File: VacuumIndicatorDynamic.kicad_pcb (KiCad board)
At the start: 2 copper layers, 151.2 x 100.4 mm, 105 parts, among them J1 Conn_01x02_Male, J2 Conn_01x03_Male, J3 Conn_01x03_Male, J4 Conn_01x03_Male, SW1 SW_DIP_x01, SW2 SW_DIP_x01, SW3 SW_DIP_x01, SW4 SW_DIP_x01, U1 AP1117-25, U2 YAAJ_BluePill

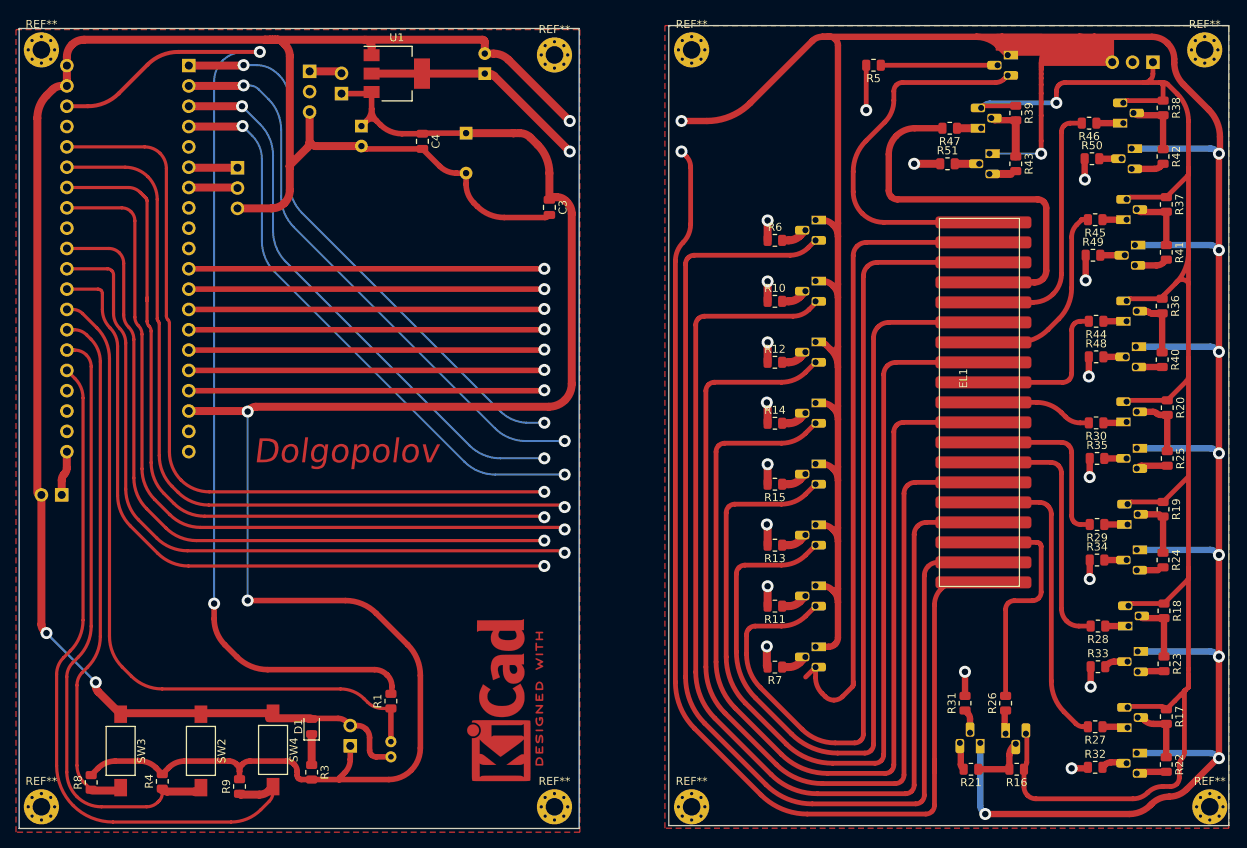
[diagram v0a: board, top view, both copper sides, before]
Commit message: major pcb update
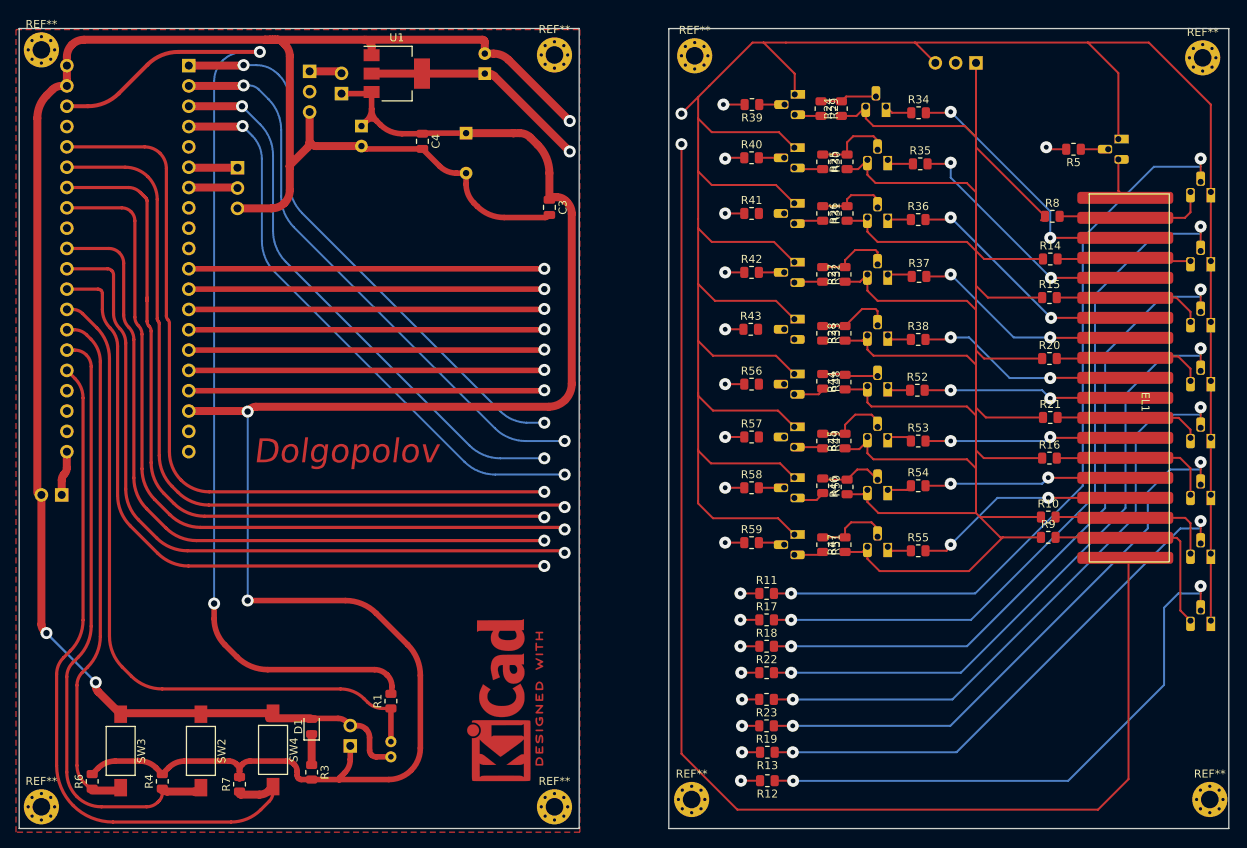
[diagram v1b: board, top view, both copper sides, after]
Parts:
- added R52: 510, Resistor_SMD:R_0805_2012Metric, F.Cu at (138.1, 68.6)
- added R53: 510, Resistor_SMD:R_0805_2012Metric, F.Cu at (138.2, 74.9)
- added R54: 510, Resistor_SMD:R_0805_2012Metric, F.Cu at (138.2, 80.5)
- added R55: 510, Resistor_SMD:R_0805_2012Metric, F.Cu at (138.2, 88.6)
- added R56: 4.7k, Resistor_SMD:R_0805_2012Metric, F.Cu at (117.3, 67.8)
- added R57: 4.7k, Resistor_SMD:R_0805_2012Metric, F.Cu at (117.3, 74.4)
- added R58: 4.7k, Resistor_SMD:R_0805_2012Metric, F.Cu at (117.3, 80.8)
- added R59: 4.7k, Resistor_SMD:R_0805_2012Metric, F.Cu at (117.3, 87.6)
- R10, R14, R15, R16, R20, R31, R32, R33, R48, R49, R50, R51: value 4.7k -> 47k
- R22, R23, R24, R25, R40, R41, R42, R43: value 47k -> 4.7k
- R26, R27, R28, R44, R45, R46, R47: value 510 -> 4.7k
- R29, R30: value 510 -> 47k
- R34, R35, R36, R37, R38: value 4.7k -> 510
- R6, R7: value 4.7k -> 10k
- R8, R9: value 10k -> 47k
- moved R8 139.4 mm to (154.9, 46.8), turned to 0 degrees
- moved R6 108.9 mm to (34.9, 117.5), turned to 90 degrees
- moved R9 105.8 mm to (154.4, 87.0), turned to 0 degrees
- moved VT16 86.9 mm to (122.7, 38.3)
- moved VT15 84.3 mm to (122.7, 31.6), turned to -90 degrees
- moved VT10 79.8 mm to (134.2, 33.1), turned to 180 degrees
- moved VT11 77.0 mm to (134.4, 39.8), turned to 180 degrees
- moved VT17 70.6 mm to (122.7, 45.2)
- moved R32 70.4 mm to (126.2, 54.1), turned to -90 degrees
- moved R24 69.3 mm to (128.6, 33.4), turned to 90 degrees
- moved R7 68.5 mm to (53.3, 117.8), turned to 90 degrees
- moved R27 64.6 mm to (129.0, 54.1), turned to 90 degrees
- moved R26 64.3 mm to (129.3, 46.5)
- moved VT5 63.9 mm to (174.8, 52.4), turned to 180 degrees
- moved R31 63.8 mm to (126.2, 46.5), turned to -90 degrees
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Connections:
- EL1 pad 1: +2V5 -> Net-(EL1-Pad1)
- EL1 pad 12: Net-(EL1-Pad12) -> /S_OUT_1
- EL1 pad 13: Net-(EL1-Pad13) -> /S_OUT_2
- EL1 pad 14: Net-(EL1-Pad14) -> /S_OUT_3
- EL1 pad 15: Net-(EL1-Pad15) -> /S_OUT_4
- EL1 pad 16: Net-(EL1-Pad16) -> /S_OUT_5
- EL1 pad 17: Net-(EL1-Pad17) -> /S_OUT_6
- EL1 pad 18: Net-(EL1-Pad18) -> /S_OUT_7
- EL1 pad 19: Net-(EL1-Pad19) -> /S_OUT_8
- EL1 pad 2: Net-(EL1-Pad2) -> +2V5
- R10 pad 1: /K2 -> +24V
- R10 pad 2: Net-(R10-Pad2) -> /S_OUT_7
- R11 pad 1: Net-(R11-Pad1) -> /S1
- R11 pad 2: /K7 -> Net-(R11-Pad2)
- R12 pad 1: /K3 -> Net-(R12-Pad1)
- R12 pad 2: Net-(R12-Pad2) -> /S8
- R13 pad 2: /K6 -> /S7
- R14 pad 1: /K4 -> +24V
- R14 pad 2: Net-(R14-Pad2) -> /S_OUT_2
- R15 pad 1: Net-(R15-Pad1) -> +24V
- R15 pad 2: /K5 -> /S_OUT_3
- R16 pad 2: Net-(R16-Pad2) -> /S_OUT_6
- R17 pad 1: +24V -> /S2
- R18 pad 1: +24V -> /S3
- R19 pad 1: +24V -> Net-(R19-Pad1)
- R19 pad 2: Net-(R19-Pad2) -> /S6
- R20 pad 2: Net-(R20-Pad2) -> /S_OUT_4
- R21 pad 1: Net-(R16-Pad2) -> +24V
- R21 pad 2: Net-(R21-Pad2) -> /S_OUT_5
- R22 pad 1: Net-(R17-Pad2) -> /S4
- R23 pad 1: Net-(R18-Pad2) -> Net-(R23-Pad1)
- R23 pad 2: Net-(R23-Pad2) -> /S5
- R24 pad 1: Net-(R19-Pad2) -> +24V
- R25 pad 1: Net-(R20-Pad2) -> +24V
- R26 pad 1: Net-(R26-Pad1) -> +24V
- R26 pad 2: /A1 -> Net-(R26-Pad2)
- R27 pad 1: Net-(R27-Pad1) -> +24V
- R27 pad 2: /A2 -> Net-(R27-Pad2)
- R28 pad 1: Net-(R28-Pad1) -> +24V
- R28 pad 2: /A3 -> Net-(R28-Pad2)
- R29 pad 1: Net-(R29-Pad1) -> Net-(R24-Pad2)
- R29 pad 2: /A4 -> Net-(R29-Pad2)
- R30 pad 1: Net-(R30-Pad1) -> Net-(R25-Pad2)
- R30 pad 2: /A5 -> Net-(R30-Pad2)
- R31 pad 1: Net-(R31-Pad1) -> Net-(R26-Pad2)
- R31 pad 2: /AU1 -> Net-(R31-Pad2)
- R32 pad 1: /AU2 -> Net-(R27-Pad2)
- R33 pad 1: /AU3 -> Net-(R28-Pad2)
- R34 pad 1: /AU4 -> Net-(R34-Pad1)
- R34 pad 2: Net-(R34-Pad2) -> /A1
- R35 pad 1: /AU5 -> Net-(R35-Pad1)
- R35 pad 2: Net-(R35-Pad2) -> /A2
- R36 pad 1: +24V -> Net-(R36-Pad1)
- R36 pad 2: Net-(R36-Pad2) -> /A3
- R37 pad 1: +24V -> Net-(R37-Pad1)
- R37 pad 2: Net-(R37-Pad2) -> /A4
- R38 pad 1: +24V -> Net-(R38-Pad1)
- R38 pad 2: Net-(R38-Pad2) -> /A5
- R39 pad 1: +24V -> Net-(R39-Pad1)
- R39 pad 2: Net-(R39-Pad2) -> /AU1
- R40 pad 1: Net-(R36-Pad2) -> /AU2
- R41 pad 1: Net-(R37-Pad2) -> /AU3
- R42 pad 1: Net-(R38-Pad2) -> /AU4
- R43 pad 1: Net-(R39-Pad2) -> /AU5
- R44 pad 1: Net-(R44-Pad1) -> +24V
- R44 pad 2: /A6 -> Net-(R44-Pad2)
- R45 pad 1: Net-(R45-Pad1) -> +24V
- R45 pad 2: /A7 -> Net-(R45-Pad2)
- R46 pad 1: Net-(R46-Pad1) -> +24V
- R46 pad 2: /A8 -> Net-(R46-Pad2)
- R47 pad 1: Net-(R47-Pad1) -> +24V
- R47 pad 2: /A9 -> Net-(R47-Pad2)
- R48 pad 1: /AU6 -> Net-(R44-Pad2)
- R49 pad 1: /AU7 -> Net-(R45-Pad2)
- R50 pad 1: /AU8 -> Net-(R46-Pad2)
- R51 pad 1: /AU9 -> Net-(R47-Pad2)
- R6 pad 1: /K1 -> /BTN3
- R6 pad 2: Net-(R6-Pad2) -> +5V
- R7 pad 1: Net-(R7-Pad1) -> /BTN1
- R7 pad 2: /K8 -> +5V
- R8 pad 1: /BTN3 -> +24V
- R8 pad 2: +5V -> /S_OUT_1
- R9 pad 1: /BTN1 -> +24V
- R9 pad 2: +5V -> /S_OUT_8
- U2 pad 1: /K3 -> /S3
- U2 pad 11: /AU9 -> /AU1
- U2 pad 12: /AU8 -> /AU2
- U2 pad 13: /AU7 -> /AU3
- U2 pad 14: /AU6 -> /AU4
- U2 pad 16: /AU4 -> /AU6
- U2 pad 17: /AU3 -> /AU7
- U2 pad 2: /K4 -> /S4
- U2 pad 29: /K8 -> /S8
- U2 pad 3: /K5 -> /S5
- U2 pad 30: /K7 -> /S7
- U2 pad 33: /AU1 -> /AU9
- U2 pad 34: /AU2 -> /AU8
- U2 pad 35: /K1 -> /S1
- U2 pad 36: /K2 -> /S2
- U2 pad 4: /K6 -> /S6
- VT1 pad 3: Net-(EL1-Pad2) -> Net-(EL1-Pad1)
- VT10 pad 1: Net-(R26-Pad1) -> Net-(R34-Pad1)
- VT10 pad 2: Net-(R16-Pad2) -> Net-(R24-Pad2)
- VT11 pad 1: Net-(R27-Pad1) -> Net-(R35-Pad1)
- VT11 pad 2: Net-(R17-Pad2) -> Net-(R25-Pad2)
- VT12 pad 1: Net-(R28-Pad1) -> Net-(R36-Pad1)
- VT12 pad 2: Net-(R18-Pad2) -> Net-(R26-Pad2)
- VT13 pad 1: Net-(R29-Pad1) -> Net-(R37-Pad1)
- VT13 pad 2: Net-(R19-Pad2) -> Net-(R27-Pad2)
- VT14 pad 1: Net-(R30-Pad1) -> Net-(R38-Pad1)
- VT14 pad 2: Net-(R20-Pad2) -> Net-(R28-Pad2)
- VT15 pad 2: Net-(R31-Pad1) -> Net-(R39-Pad1)
- VT15 pad 3: Net-(R21-Pad2) -> Net-(R29-Pad2)
- VT16 pad 2: Net-(R32-Pad2) -> Net-(R40-Pad2)
- VT16 pad 3: Net-(R22-Pad2) -> Net-(R30-Pad2)
- VT17 pad 2: Net-(R33-Pad2) -> Net-(R41-Pad2)
- VT17 pad 3: Net-(R23-Pad2) -> Net-(R31-Pad2)
- VT18 pad 2: Net-(R34-Pad2) -> Net-(R42-Pad2)
- VT18 pad 3: Net-(R24-Pad2) -> Net-(R32-Pad2)
- VT19 pad 2: Net-(R35-Pad2) -> Net-(R43-Pad2)
- VT19 pad 3: Net-(R25-Pad2) -> Net-(R33-Pad2)
- VT2 pad 2: Net-(R6-Pad2) -> Net-(R11-Pad2)
- VT2 pad 3: Net-(EL1-Pad12) -> /S_OUT_1
- VT20 pad 1: Net-(R44-Pad1) -> Net-(R52-Pad1)
- VT20 pad 2: Net-(R36-Pad2) -> Net-(R44-Pad2)
- VT21 pad 1: Net-(R45-Pad1) -> Net-(R53-Pad1)
- VT21 pad 2: Net-(R37-Pad2) -> Net-(R45-Pad2)
- VT22 pad 1: Net-(R46-Pad1) -> Net-(R54-Pad1)
- VT22 pad 2: Net-(R38-Pad2) -> Net-(R46-Pad2)
- VT23 pad 1: Net-(R47-Pad1) -> Net-(R55-Pad1)
- VT23 pad 2: Net-(R39-Pad2) -> Net-(R47-Pad2)
- VT24 pad 2: Net-(R48-Pad2) -> Net-(R56-Pad2)
- VT24 pad 3: Net-(R40-Pad2) -> Net-(R48-Pad2)
- VT25 pad 2: Net-(R49-Pad2) -> Net-(R57-Pad2)
- VT25 pad 3: Net-(R41-Pad2) -> Net-(R49-Pad2)
- VT26 pad 2: Net-(R50-Pad2) -> Net-(R58-Pad2)
- VT26 pad 3: Net-(R42-Pad2) -> Net-(R50-Pad2)
- VT27 pad 2: Net-(R51-Pad2) -> Net-(R59-Pad2)
- VT27 pad 3: Net-(R43-Pad2) -> Net-(R51-Pad2)
- VT3 pad 2: Net-(R7-Pad1) -> Net-(R12-Pad1)
- VT3 pad 3: Net-(EL1-Pad19) -> /S_OUT_8
- VT4 pad 2: Net-(R10-Pad2) -> Net-(R13-Pad1)
- VT4 pad 3: Net-(EL1-Pad13) -> /S_OUT_7
- VT5 pad 2: Net-(R11-Pad1) -> Net-(R17-Pad2)
- VT5 pad 3: Net-(EL1-Pad18) -> /S_OUT_2
- VT6 pad 2: Net-(R12-Pad2) -> Net-(R18-Pad2)
- VT6 pad 3: Net-(EL1-Pad14) -> /S_OUT_3
- VT7 pad 2: Net-(R13-Pad1) -> Net-(R19-Pad1)
- VT7 pad 3: Net-(EL1-Pad17) -> /S_OUT_6
- VT8 pad 2: Net-(R14-Pad2) -> Net-(R22-Pad2)
- VT8 pad 3: Net-(EL1-Pad15) -> /S_OUT_4
- VT9 pad 2: Net-(R15-Pad1) -> Net-(R23-Pad1)
- VT9 pad 3: Net-(EL1-Pad16) -> /S_OUT_5
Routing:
- net Net-(EL1-Pad12): track 138.9 -> 0.00 mm
- net Net-(EL1-Pad13): track 131.8 -> 0.00 mm
- net Net-(EL1-Pad14): track 123.9 -> 0.00 mm
- net Net-(EL1-Pad15): track 119.2 -> 0.00 mm
- net Net-(EL1-Pad16): track 118.4 -> 0.00 mm
- net Net-(EL1-Pad17): track 110.9 -> 0.00 mm
- net Net-(EL1-Pad18): track 106.9 -> 0.00 mm
- net /K1: track 102.2 -> 0.00 mm, vias 2 -> 0
- net /S1: track 0.00 -> 102.0 mm, vias 0 -> 2
- net /K2: track 101.6 -> 0.00 mm, vias 2 -> 0
- net /S2: track 0.00 -> 101.4 mm, vias 0 -> 2
- net GND: track 688.1 -> 591.5 mm, vias 13 -> 4
- net Net-(R11-Pad2): track 0.00 -> 96.6 mm, vias 0 -> 2
- net /K7: track 94.8 -> 0.00 mm, vias 2 -> 0
- net /S7: track 0.00 -> 94.6 mm, vias 0 -> 2
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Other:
- board size 151.2 x 100.4 mm -> 151.2 x 100 mm
